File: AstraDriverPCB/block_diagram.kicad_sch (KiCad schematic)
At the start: 32 parts, among them CN1 JST VH 8 PIN, CN2 JST VH 2 PIN, CN3 JST VH 2 PIN, CN4 JST VH 2 PIN, CN5 JST VH 2 PIN

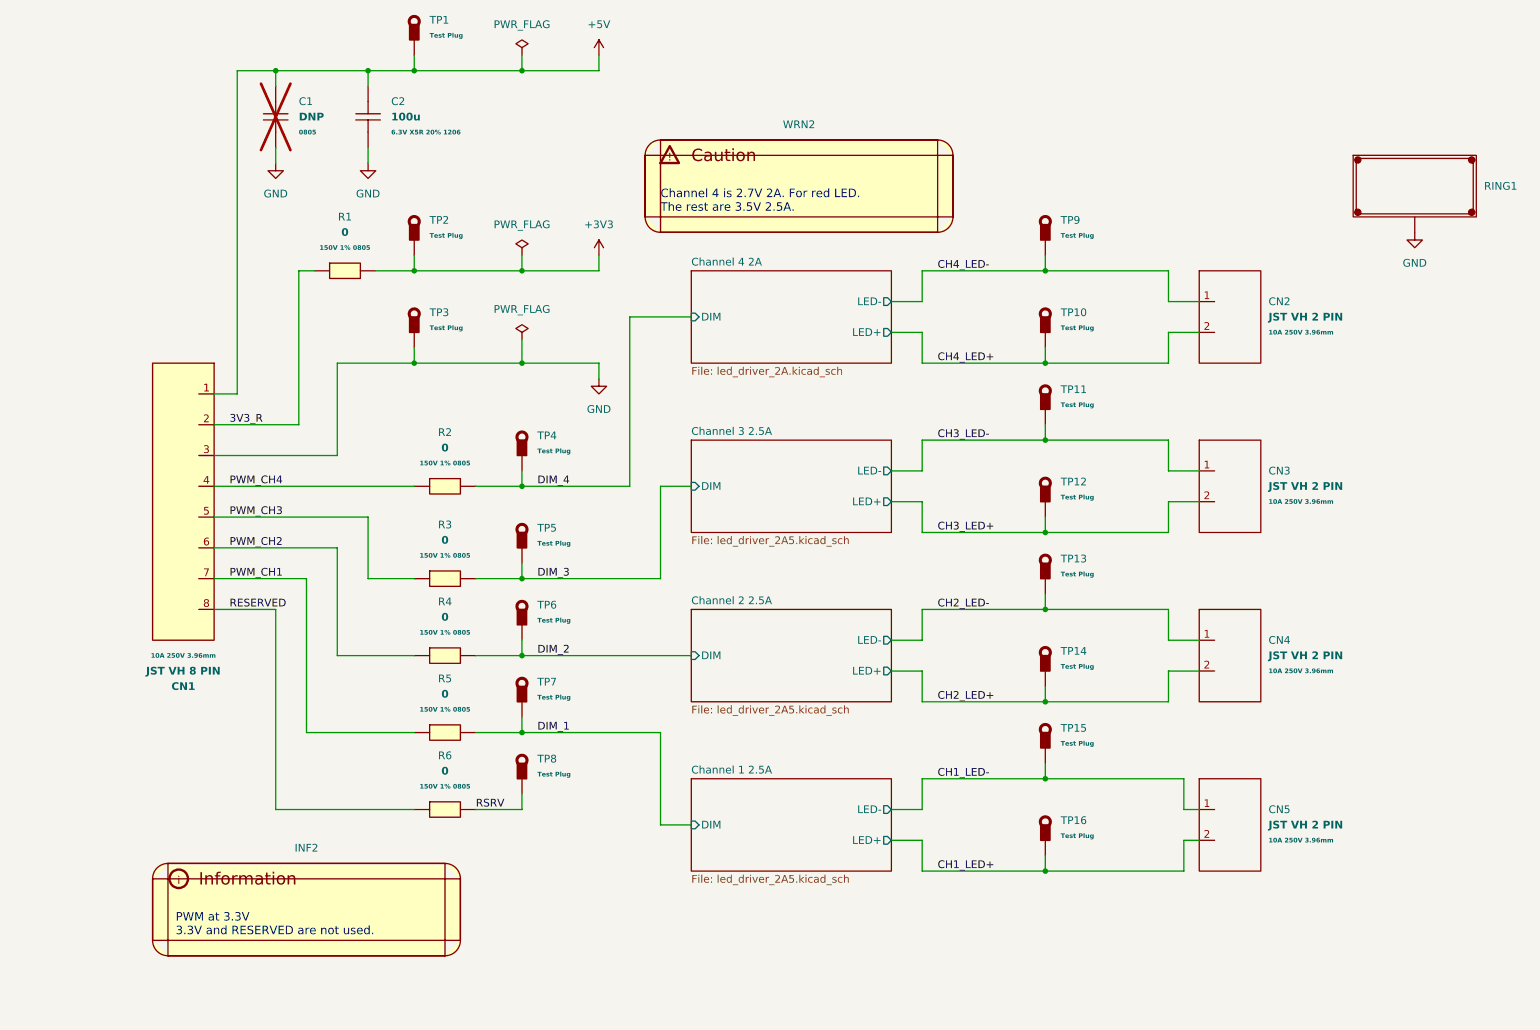
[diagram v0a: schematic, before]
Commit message: New layout in progress
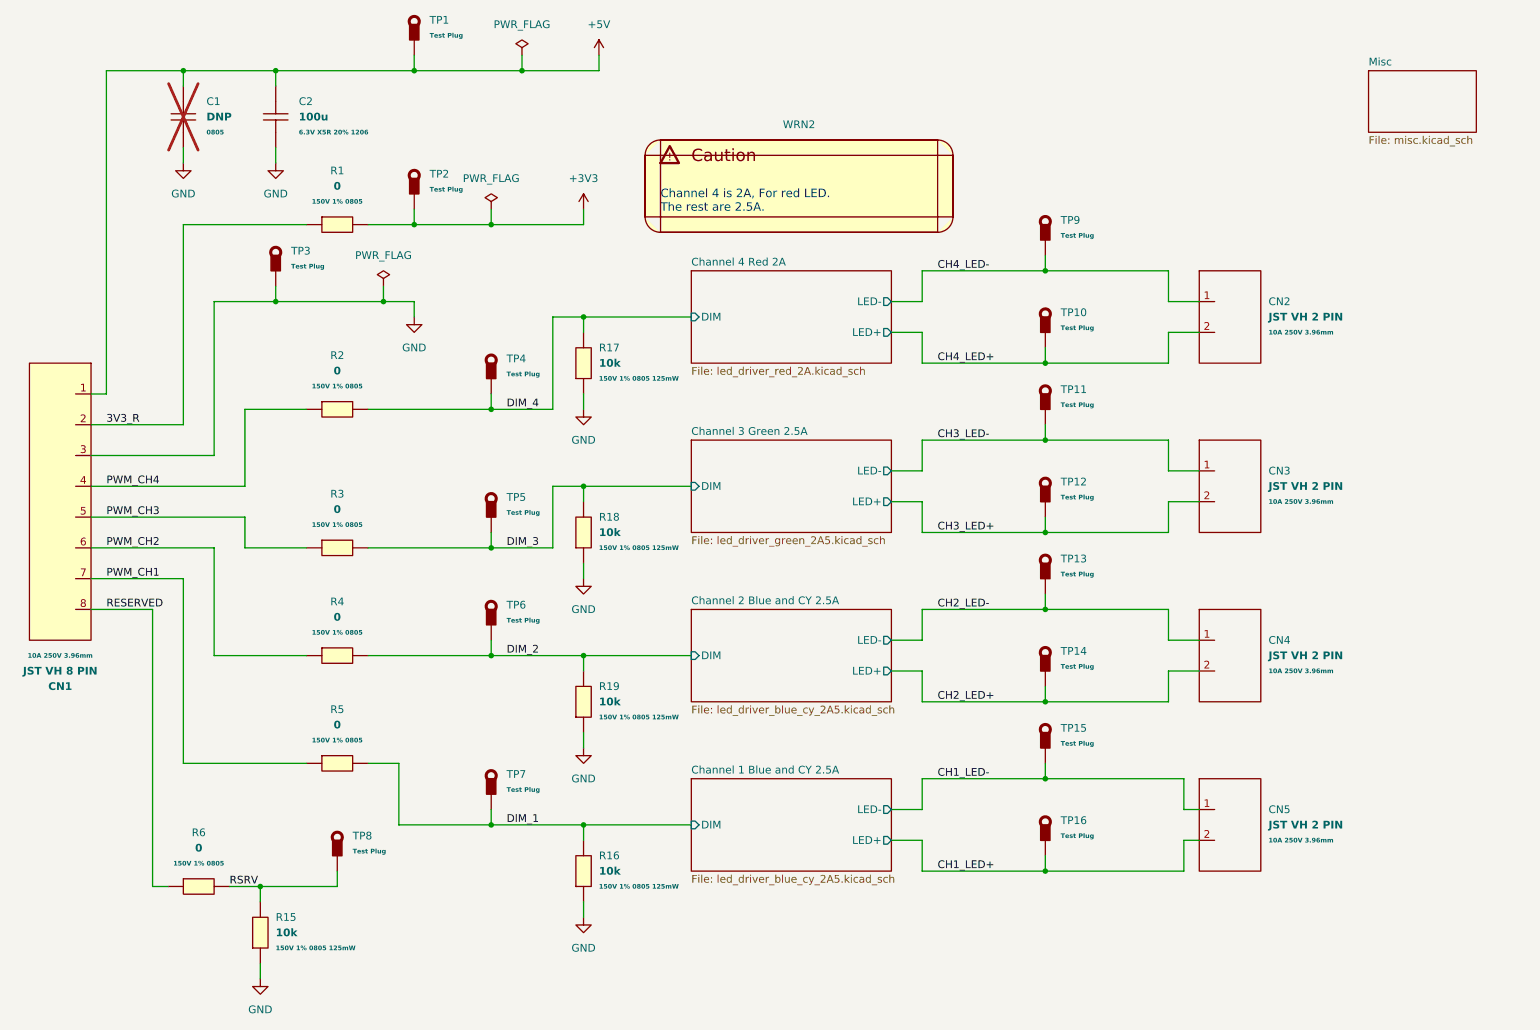
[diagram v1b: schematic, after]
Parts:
- removed INF2: ~, symbol LiveAstra:Information_Box
- removed RING1: ~, LiveAstra:AstraControl_Ground_Ring, symbol LiveAstra:AstraControl_Ground_Ring
- added R15, R16, R17, R18, R19: 10k, LiveAstra:R_0805_2012Metric_Pad1.20x1.40mm_HandSolder, symbol LiveAstra:R_10kOhm_0805_125mW
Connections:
- net DIM_1: now also R16.2
- net DIM_2: now also R19.2
- net DIM_3: now also R18.2
- net DIM_4: now also R17.2
- net GND: now also R15.1, R16.1, R17.1, R18.1, R19.1
- net RSRV: now also R15.2
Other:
- sheet Channel 2 2.5A renamed Channel 2 Blue and CY 2.5A
- sheet Channel 3 2.5A renamed Channel 3 Green 2.5A
- sheet Channel 4 2A renamed Channel 4 Red 2A
- removed sheet Channel 1 2.5A
- added sheet Channel 1 Blue and CY 2.5A (led_driver_blue_cy_2A5.kicad_sch)
- added sheet Misc (misc.kicad_sch)
- sheet Channel 2 Blue and CY 2.5A: file led_driver_2A5.kicad_sch -> led_driver_blue_cy_2A5.kicad_sch
- sheet Channel 3 Green 2.5A: file led_driver_2A5.kicad_sch -> led_driver_green_2A5.kicad_sch
- sheet Channel 4 Red 2A: file led_driver_2A.kicad_sch -> led_driver_red_2A.kicad_sch
- note added: "Channel 4 is 2A, For red LED. The rest are 2.5A."
- note removed: "Channel 4 is 2.7V 2A. For red LED. The rest are 3.5V 2.5A."
- note removed: "PWM at 3.3V 3.3V and RESERVED are not used."
- moved on the sheet: C1, C2, CN1, R1, R2, R3, R4, R5, R6, TP2, TP3, TP4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
